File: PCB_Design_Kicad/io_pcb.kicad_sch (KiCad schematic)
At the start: 17 parts, among them J12 front bottom, J14 front top, J15 SD-50BV, J16 midi, J3 Voct_A, J4 Trig_A, J5 Vel_A, J6 Voct_B, J7 Trig_B, J8 Vel_B, J9 adv_clock_out, SW1 re-sync, SW2 midi learn, SW3 seq. mode

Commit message: more bom
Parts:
- J15: footprint SamacSys_Parts:SD-50BV -> WeirdVibes_Eurorack:CUI SD-50BV MIDI DIN-5
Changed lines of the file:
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@@
+			)
+		)
+		(property "Comment" ""
+			(at 39.37 67.945 0)
+			(effects
+				(font
+					(size 1.27 1.27)
+				)
+				(hide yes)
 			)
 		)
@@
 			)
 		)
+		(property "Comment" ""
+			(at 152.4 75.565 0)
+			(effects
+				(font
+					(size 1.27 1.27)
+				)
+				(hide yes)
+			)
+		)
 		(pin "S"
 		)
@@
 			)
 		)
+		(property "Comment" ""
+			(at 53.975 55.245 0)
+			(effects
+				(font
+					(size 1.27 1.27)
+				)
+				(hide yes)
+			)
+		)
 		(pin "2"
 		)
@@
 			)
 		)
+		(property "Comment" ""
+			(at 152.4 38.1 0)
+			(effects
+				(font
+					(size 1.27 1.27)
+				)
+				(hide yes)
+			)
+		)
 		(pin "S"
 		)
@@
 			)
 		)
-		(property "Footprint" "SamacSys_Parts:SD-50BV"
+		(property "Footprint" "WeirdVibes_Eurorack:CUI SD-50BV MIDI DIN-5"
 			(at 141.605 133.985 0)
 			(effects
@@
 		)
 		(property "Price (single)" ""
+			(at 125.095 136.525 0)
+			(effects
+				(font
+					(size 1.27 1.27)
+				)
+				(hide yes)
+			)
+		)
+		(property "Comment" ""
 			(at 125.095 136.525 0)
 			(effects
@@
 			)
 		)
+		(property "Comment" ""
+			(at 152.4 23.495 0)
+			(effects
+				(font
+					(size 1.27 1.27)
+				)
+				(hide yes)
+			)
+		)
 		(pin "S"
 		)
@@
 		)
 		(property "Price (single)" ""
+			(at 36.83 76.2 0)
+			(effects
+				(font
+					(size 1.27 1.27)
+				)
+				(hide yes)
+			)
+		)
+		(property "Comment" ""
 			(at 36.83 76.2 0)
 			(effects
@@
 			)
 		)
+		(property "Comment" ""
+			(at 152.4 92.71 0)
+			(effects
+				(font
+					(size 1.27 1.27)
+				)
+				(hide yes)
+			)
+		)
 		(pin "S"
 		)
@@
 			)
 		)
+		(property "Comment" ""
+			(at 206.375 64.135 0)
+			(effects
+				(font
+					(size 1.27 1.27)
+				)
+				(hide yes)
+			)
+		)
 		(pin "2"
 		)
@@
 			)
 		)
+		(property "Comment" ""
+			(at 57.15 34.29 0)
+			(effects
+				(font
+					(size 1.27 1.27)
+				)
+				(hide yes)
+			)
+		)
 		(pin "S"
 		)
@@
 		)
 		(property "Price (single)" ""
+			(at 149.225 54.61 0)
+			(effects
+				(font
+					(size 1.27 1.27)
+				)
+				(hide yes)
+			)
+		)
+		(property "Comment" ""
 			(at 149.225 54.61 0)
 			(effects
@@
 			)
 		)
+		(property "Comment" ""
+			(at 152.4 108.585 0)
+			(effects
+				(font
+					(size 1.27 1.27)
+				)
+				(hide yes)
+			)
+		)
 		(pin "S"
 		)
@@
 			)
 		)
+		(property "Comment" ""
+			(at 166.37 136.525 0)
+			(effects
+				(font
+					(size 1.27 1.27)
+				)
+				(hide yes)
+			)
+		)
 		(pin "3"
 		)
@@
 			)
 		)
+		(property "Comment" ""
+			(at 51.435 113.03 0)
+			(effects
+				(font
+					(size 1.27 1.27)
+				)
+				(hide yes)
+			)
+		)
 		(pin "2"
 		)
@@
 		)
 		(property "Price (single)" ""
+			(at 57.785 90.805 0)
+			(effects
+				(font
+					(size 1.27 1.27)
+				)
+				(hide yes)
+			)
+		)
+		(property "Comment" ""
 			(at 57.785 90.805 0)
 			(effects
@@
 			)
 		)
+		(property "Comment" ""
+			(at 57.15 20.955 0)
+			(effects
+				(font
+					(size 1.27 1.27)
+				)
+				(hide yes)
+			)
+		)
 		(pin "S"
 		)
@@
 			(at 102.87 80.01 0)
 			(effects
+				(font
+					(size 1.27 1.27)
+				)
+				(hide yes)
+			)
+		)
+		(property "Comment" ""
+			(at 102.87 80.01 0)
+			(effects

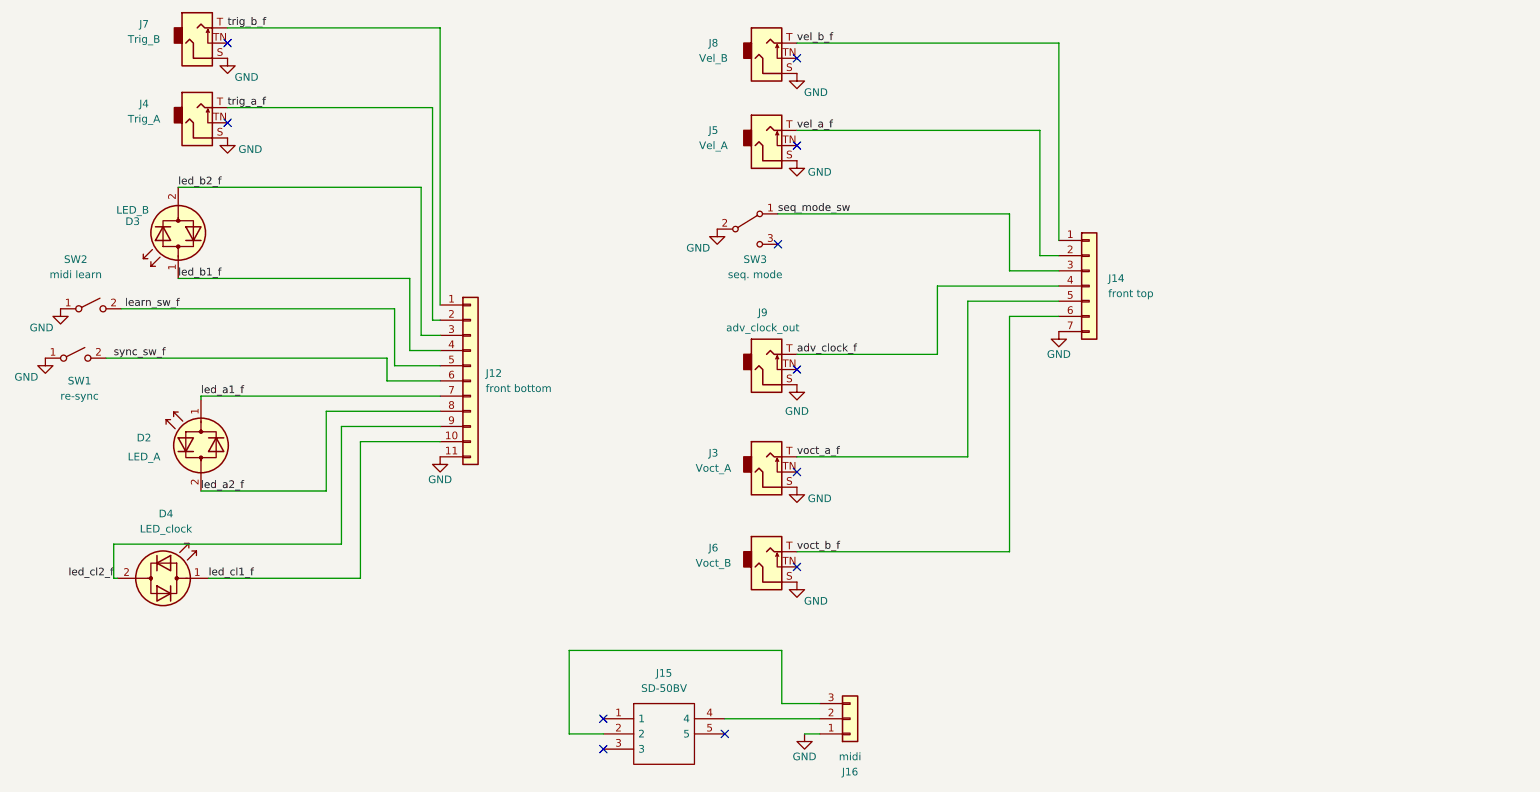
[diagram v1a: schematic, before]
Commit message: pcb
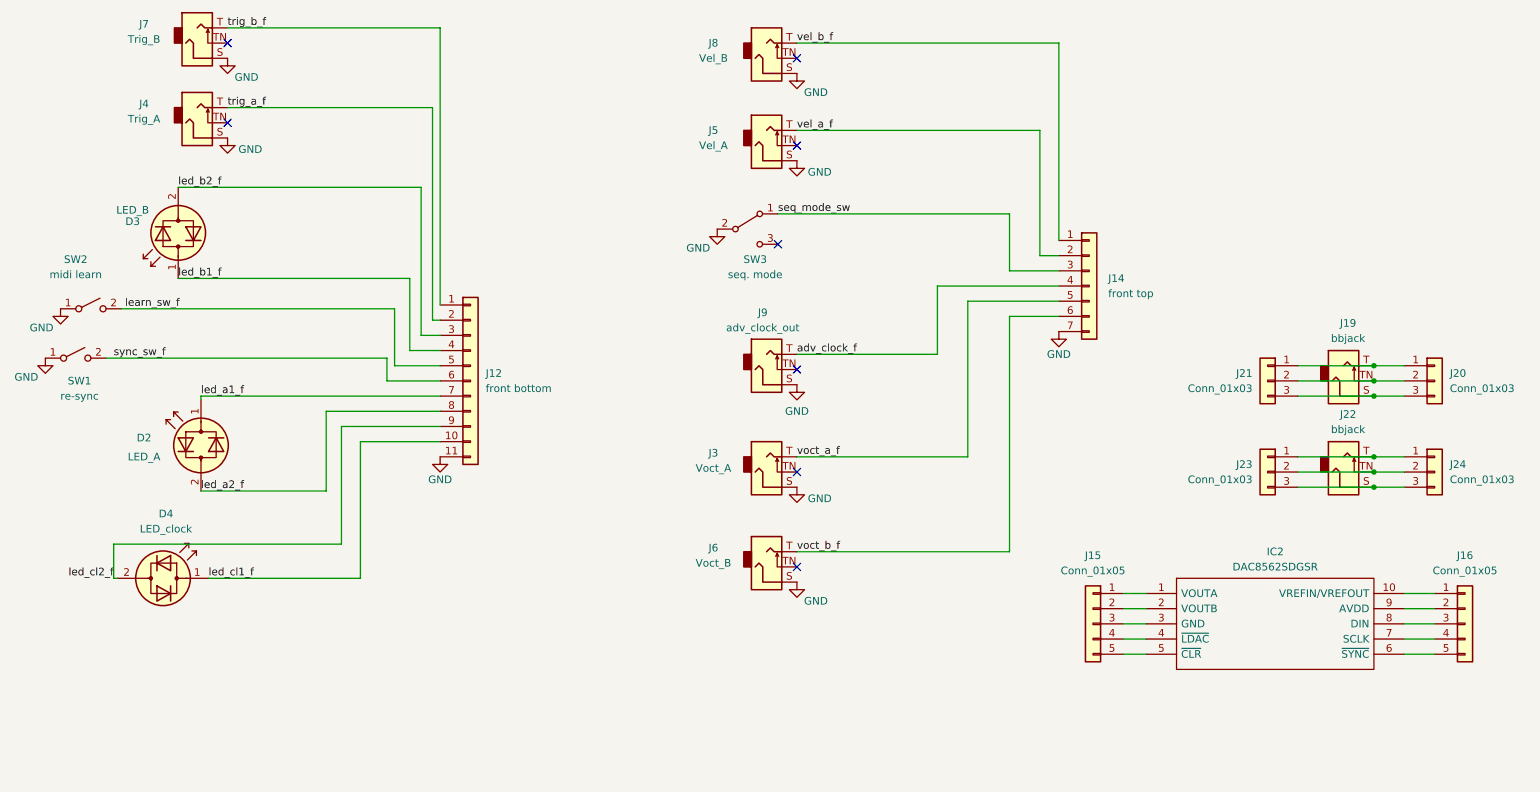
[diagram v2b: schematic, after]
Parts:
- removed J15: SD-50BV, WeirdVibes_Eurorack:CUI SD-50BV MIDI DIN-5, symbol SamacSys_Parts:SD-50BV
- removed J16: midi, Connector_PinSocket_2.54mm:PinSocket_1x03_P2.54mm_Vertical, symbol Connector_Generic:Conn_01x03
- added IC2: DAC8562SDGSR, SamacSys_Parts:SOP50P490X110-10N, symbol SamacSys_Parts:DAC8562SDGSR
- added J15, J16: Conn_01x05, Connector_PinHeader_2.54mm:PinHeader_1x05_P2.54mm_Vertical, symbol Connector_Generic:Conn_01x05
- added J19, J22: bbjack, WeirdVibes:Thonkiconn, symbol WeirdVibes_Eurorack:AudioJack_Switch
- added J20, J21, J23, J24: Conn_01x03, Connector_PinHeader_2.54mm:PinHeader_1x03_P2.54mm_Vertical, symbol Connector_Generic:Conn_01x03
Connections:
- new net: J19.S, J20.3 (Pin_3), J21.3 (Pin_3)
- new net: J19.T, J20.1 (Pin_1), J21.1 (Pin_1)
- new net: J19.TN, J20.2 (Pin_2), J21.2 (Pin_2)
- new net: IC2.1 (VOUTA), J15.1 (Pin_1)
- new net: IC2.10 (VREFIN/VREFOUT), J16.1 (Pin_1)
- new net: IC2.2 (VOUTB), J15.2 (Pin_2)
- new net: IC2.3 (GND), J15.3 (Pin_3)
- new net: IC2.4 (~{LDAC}), J15.4 (Pin_4)
- new net: IC2.5 (~{CLR}), J15.5 (Pin_5)
- new net: IC2.6 (~{SYNC}), J16.5 (Pin_5)
- new net: IC2.7 (SCLK), J16.4 (Pin_4)
- new net: IC2.8 (DIN), J16.3 (Pin_3)
- new net: IC2.9 (AVDD), J16.2 (Pin_2)
- new net: J22.T, J23.1 (Pin_1), J24.1 (Pin_1)
- new net: J22.TN, J23.2 (Pin_2), J24.2 (Pin_2)
- new net: J22.S, J23.3 (Pin_3), J24.3 (Pin_3)
- no-connect marks 11 -> 8

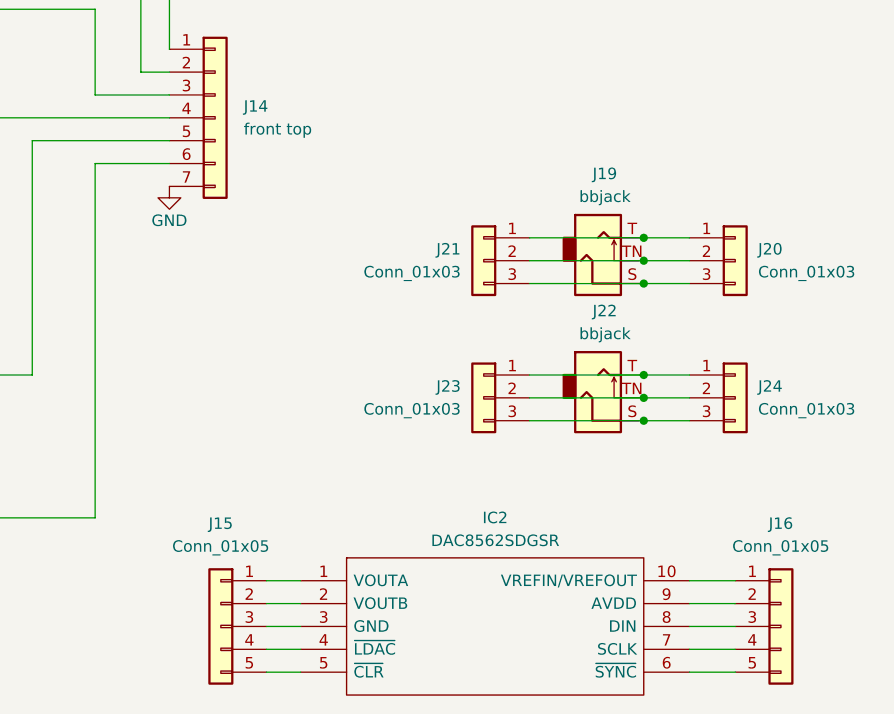
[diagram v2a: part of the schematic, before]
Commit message: pcb versions sent to jlcpcb
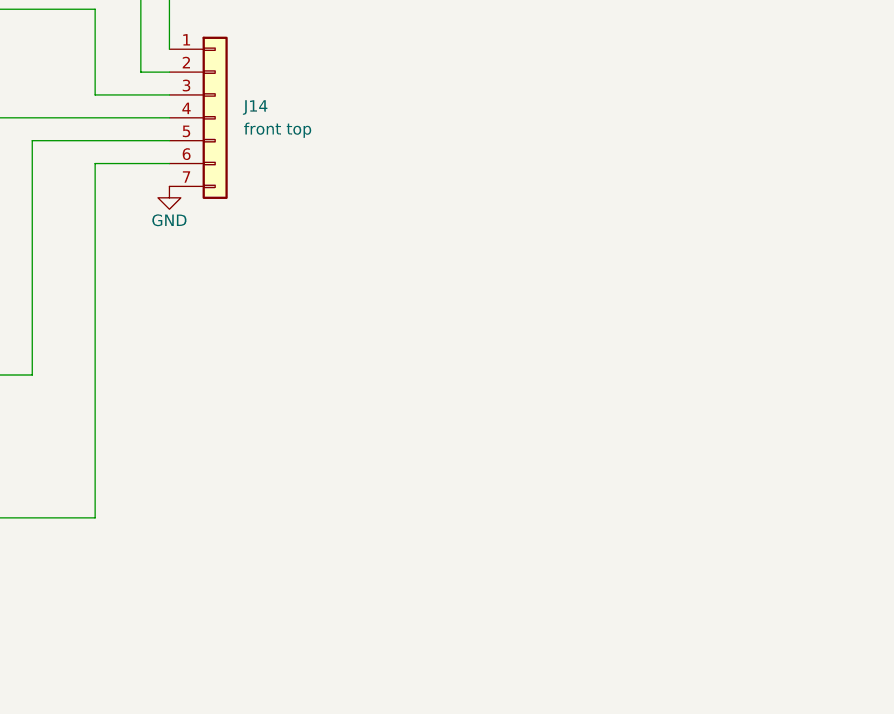
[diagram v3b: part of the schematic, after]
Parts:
- removed IC2: DAC8562SDGSR, SamacSys_Parts:SOP50P490X110-10N, symbol SamacSys_Parts:DAC8562SDGSR
- removed J15, J16: Conn_01x05, Connector_PinHeader_2.54mm:PinHeader_1x05_P2.54mm_Vertical, symbol Connector_Generic:Conn_01x05
- removed J19, J22: bbjack, WeirdVibes:Thonkiconn, symbol WeirdVibes_Eurorack:AudioJack_Switch
- removed J20, J21, J23, J24: Conn_01x03, Connector_PinHeader_2.54mm:PinHeader_1x03_P2.54mm_Vertical, symbol Connector_Generic:Conn_01x03
